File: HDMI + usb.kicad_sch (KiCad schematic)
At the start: 37 parts, among them J2 Micro_SD_Card_Det2, J3 USB_C_Receptacle_USB2.0_16P, J4 USB_C_Receptacle_USB2.0_16P, J5 HDMI_C_1.4, Q1 2N7002, SW1 SW_Push, SW2 SW_Push, SW3 SW_Push, SW4 SW_Push, U3 SPI-EEPROM

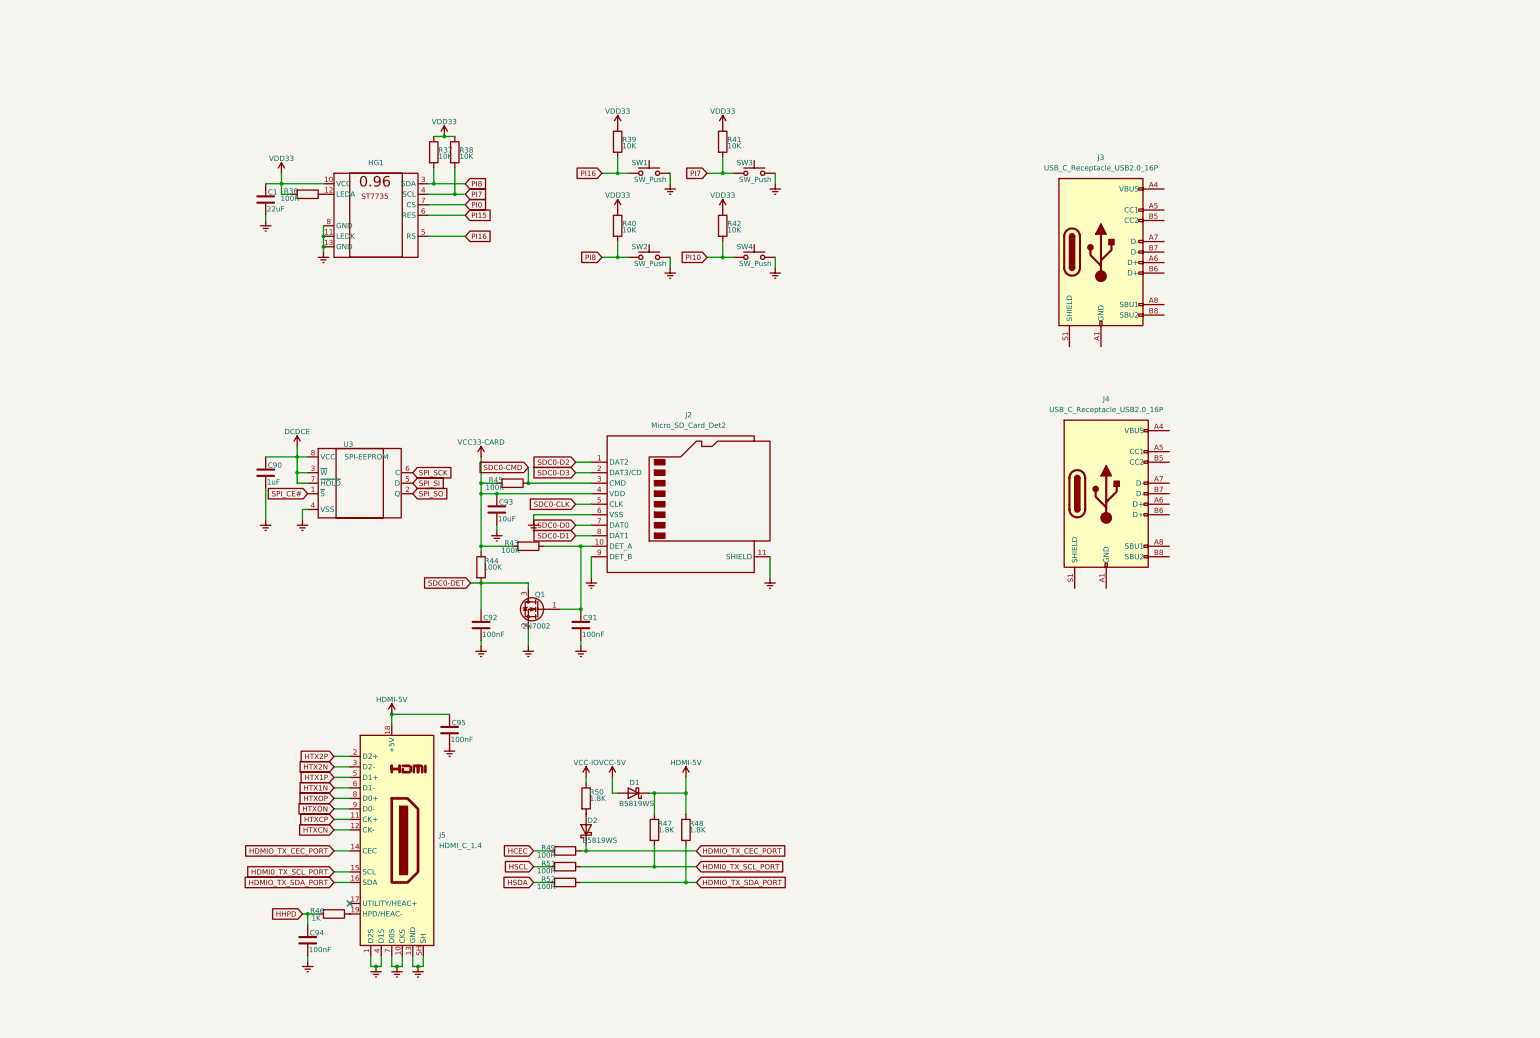
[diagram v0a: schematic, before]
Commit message: Схема закончена, часть компонентов расставлена на плате
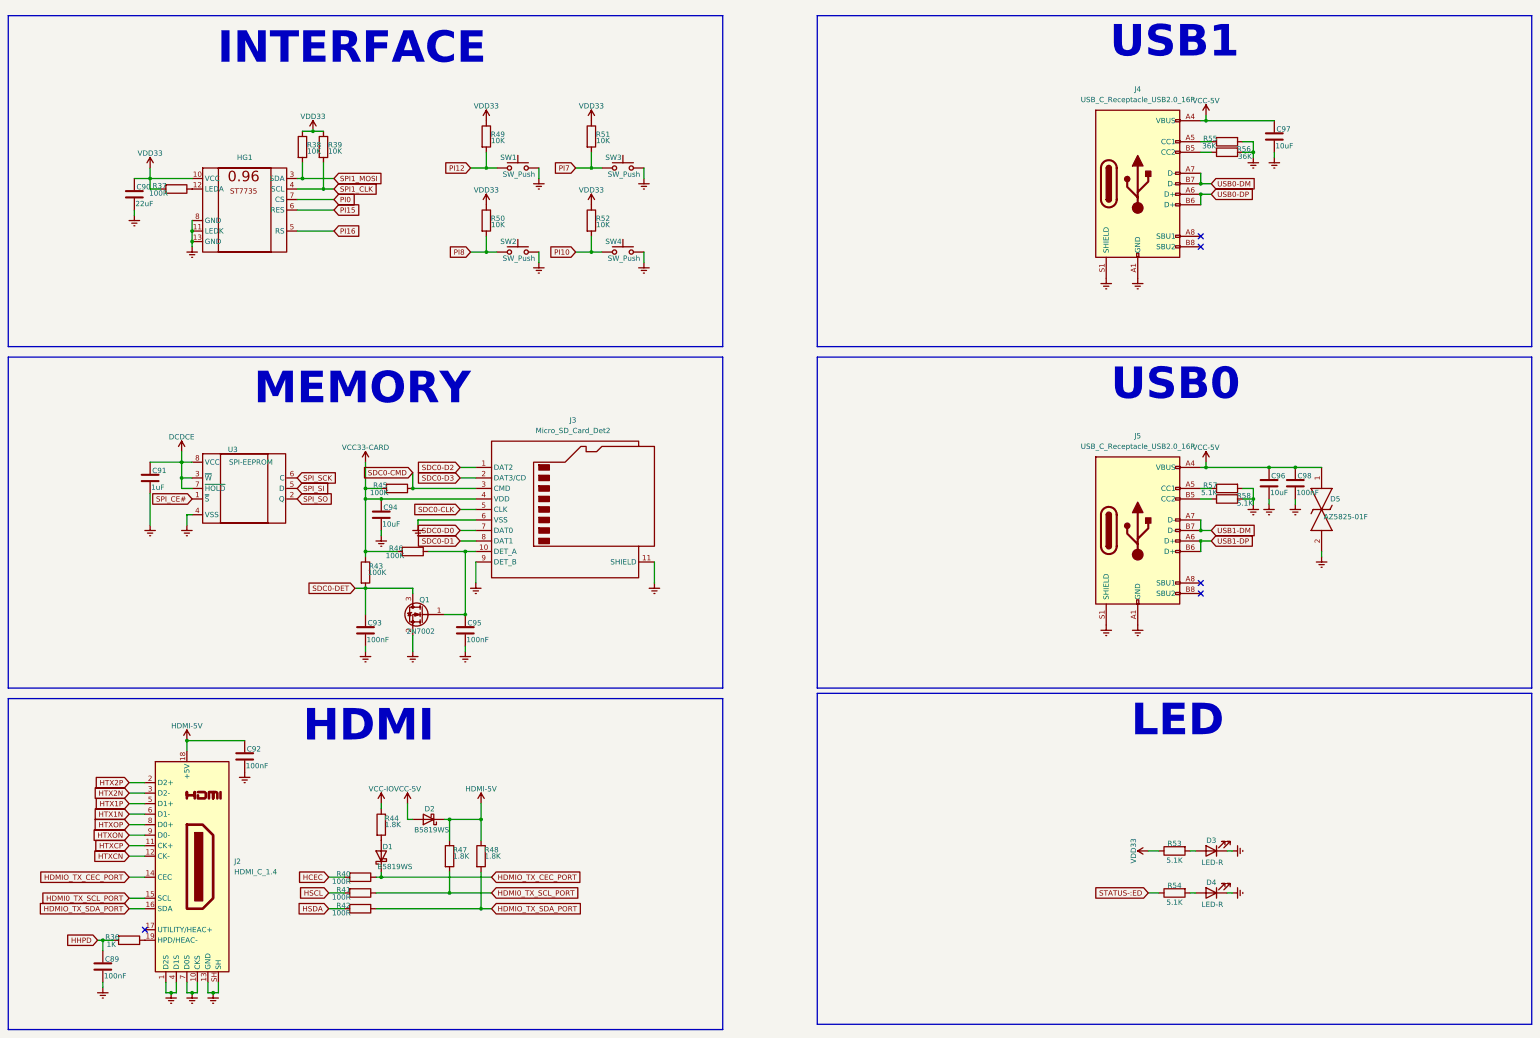
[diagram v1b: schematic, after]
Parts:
- removed J4: USB_C_Receptacle_USB2.0_16P, Connector_USB:USB_C_Receptacle_G-Switch_GT-USB-7010ASV, symbol Connector:USB_C_Receptacle_USB2.0_16P
- added C96, C97: 10uF, Capacitor_SMD:C_0402_1005Metric, symbol Device:C
- added C98: 100nF, Capacitor_SMD:C_0402_1005Metric, symbol Device:C
- added D3, D4: LED-R, LED_SMD:LED_0402_1005Metric, symbol Device:LED
- added D5: AZ5825-01F, ESD:AZ582501F, symbol ESD:AZ5825-01F
- added J5: USB_C_Receptacle_USB2.0_16P, Connector_USB:USB_C_Receptacle_G-Switch_GT-USB-7010ASV, symbol Connector:USB_C_Receptacle_USB2.0_16P
- added R53, R54, R57, R58: 5.1K, Resistor_SMD:R_0402_1005Metric, symbol Device:R
- added R55, R56: 36K, Resistor_SMD:R_0402_1005Metric, symbol Device:R
- renumbered C94 to C89, C1 to C90, C90 to C91, C95 to C92, C92 to C93, C93 to C94, C91 to C95, D2 to D1, D1 to D2, J5 to J2, J2 to J3, J3 to J4, R46 to R36, R36 to R37, R37 to R38, R38 to R39, R49 to R40, R51 to R41, R52 to R42, R44 to R43, R50 to R44, R43 to R46, R39 to R49, R40 to R50, R41 to R51, R42 to R52
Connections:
- net Earth: now also J4.A1 (GND), J4.A12 (GND), J4.B1 (GND), J4.B12 (GND), J4.S1 (SHIELD), C96.2, C97.2, C98.2, D3.1 (K), D4.1 (K), D5.2, J5.A1 (GND), J5.A12 (GND), J5.B1 (GND), J5.B12 (GND), J5.S1 (SHIELD), R55.2, R56.2, R57.2, R58.2
- net PI16: no longer R49.2, SW1.1
- net PI7: no longer HG1.4 (SCL), R39.2
- net PI8: no longer HG1.3 (SDA), R38.2
- net VCC-5V: now also J4.A4 (VBUS), J4.A9 (VBUS), J4.B4 (VBUS), J4.B9 (VBUS), C96.1, C97.1, C98.1, D5.1, J5.A4 (VBUS), J5.A9 (VBUS), J5.B4 (VBUS), J5.B9 (VBUS)
- net VDD33: now also R53.1
- net at J4.A5 (CC1): now also R55.1
- net USB0-DP: now reaches J4.A6 (D+)
- net USB0-DP: now also J4.B6 (D+)
- net USB0-DM: now reaches J4.A7 (D-)
- net USB0-DM: now also J4.B7 (D-)
- net at J4.B5 (CC2): now also R56.1
- new net: J5.A5 (CC1), R57.1
- new net: J5.B5 (CC2), R58.1
- new net: D4.2 (A), R54.2
- new net: D3.2 (A), R53.2
- new net PI12: R49.2, SW1.1
- new net SPI1_CLK: HG1.4 (SCL), R39.2
- new net SPI1_MOSI: HG1.3 (SDA), R38.2
- new net STATUS-:ED: R54.1
- new net USB1-DM: J5.A7 (D-), J5.B7 (D-)
- new net USB1-DP: J5.A6 (D+), J5.B6 (D+)
- no-connect marks 1 -> 5
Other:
- note added: "HDMI"
- note added: "INTERFACE"
- note added: "LED"
- note added: "MEMORY"
- note added: "USB0"
- note added: "USB1"
- moved on the sheet: C89, C90, C91, C92, C93, C94, C95, D1, D2, HG1, J2, J3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
